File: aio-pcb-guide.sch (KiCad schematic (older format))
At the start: 12 parts

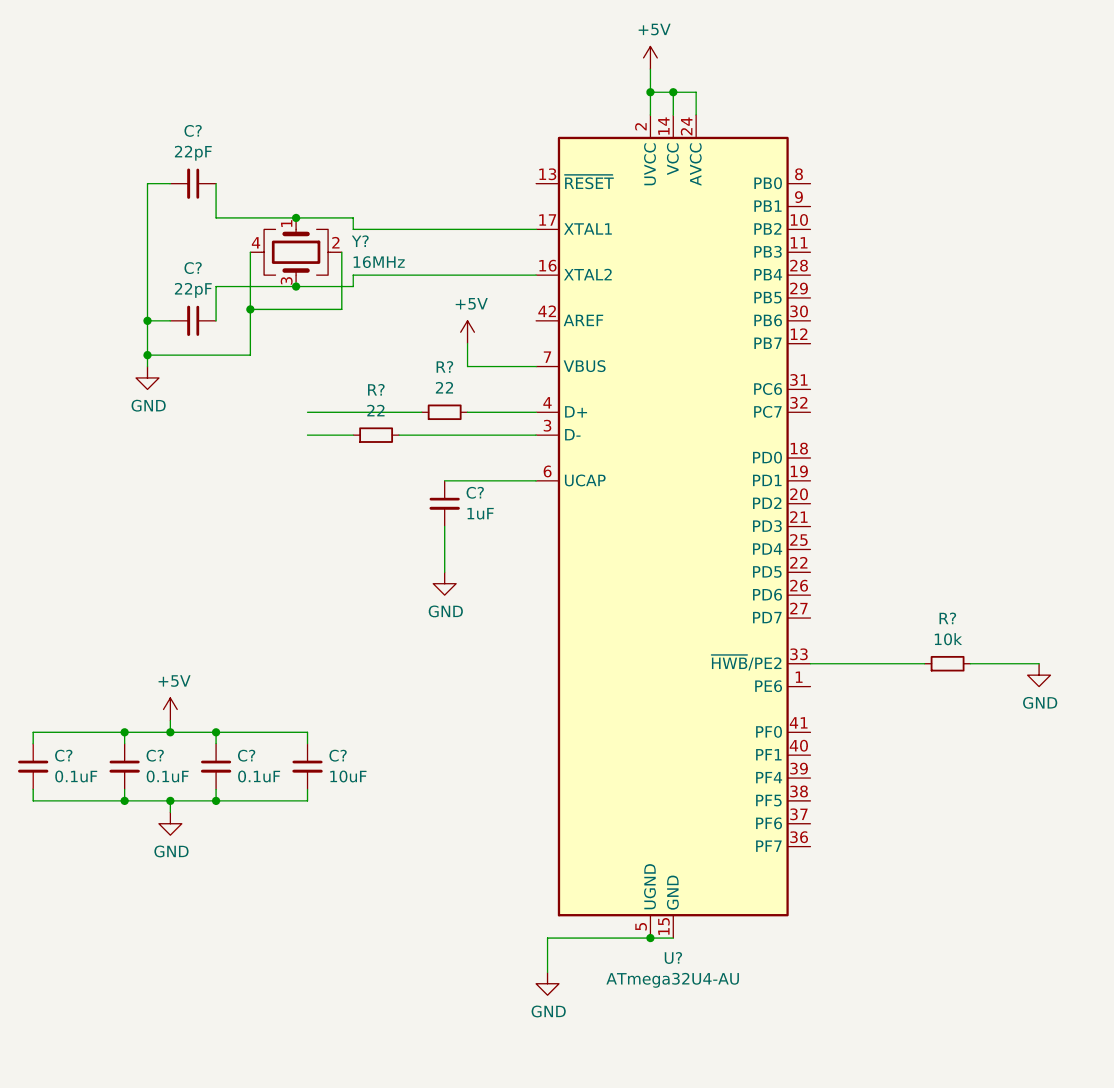
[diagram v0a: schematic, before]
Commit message: completed MCU
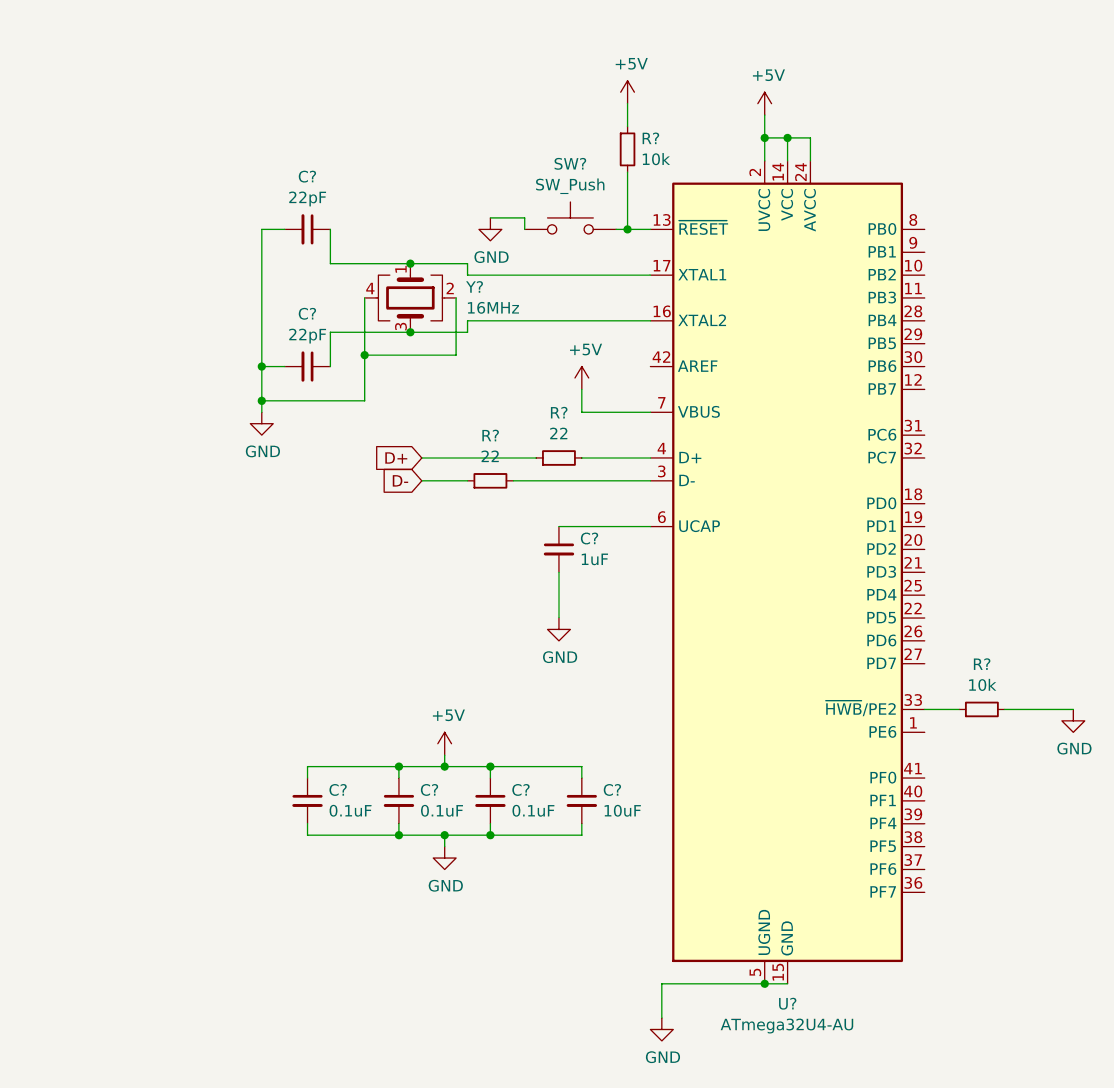
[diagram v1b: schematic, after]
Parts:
- added R?: 10k, symbol Device:R_Small
- added SW?: SW_Push, symbol Switch:SW_Push
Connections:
- net labels added: D+, D-
- wire segments 57 -> 63
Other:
- moved on the sheet: C?, R?, U?, Y?
